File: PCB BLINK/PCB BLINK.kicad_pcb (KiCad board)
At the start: 2 copper layers, 74.9 x 74.9 mm, 6 parts, among them U2 HC-SR04, U3 ER_OLEDM0.91_1x-I2C

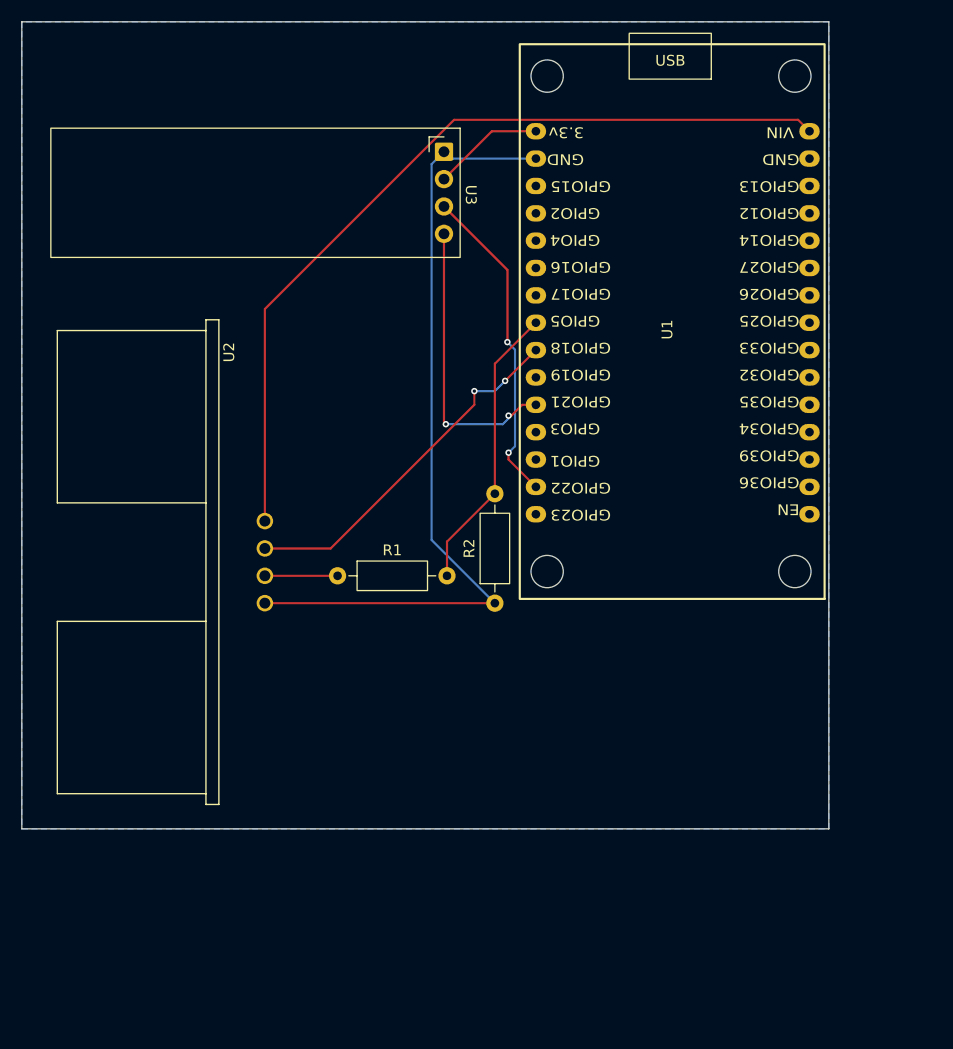
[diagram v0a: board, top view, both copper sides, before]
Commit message: case and pcb production
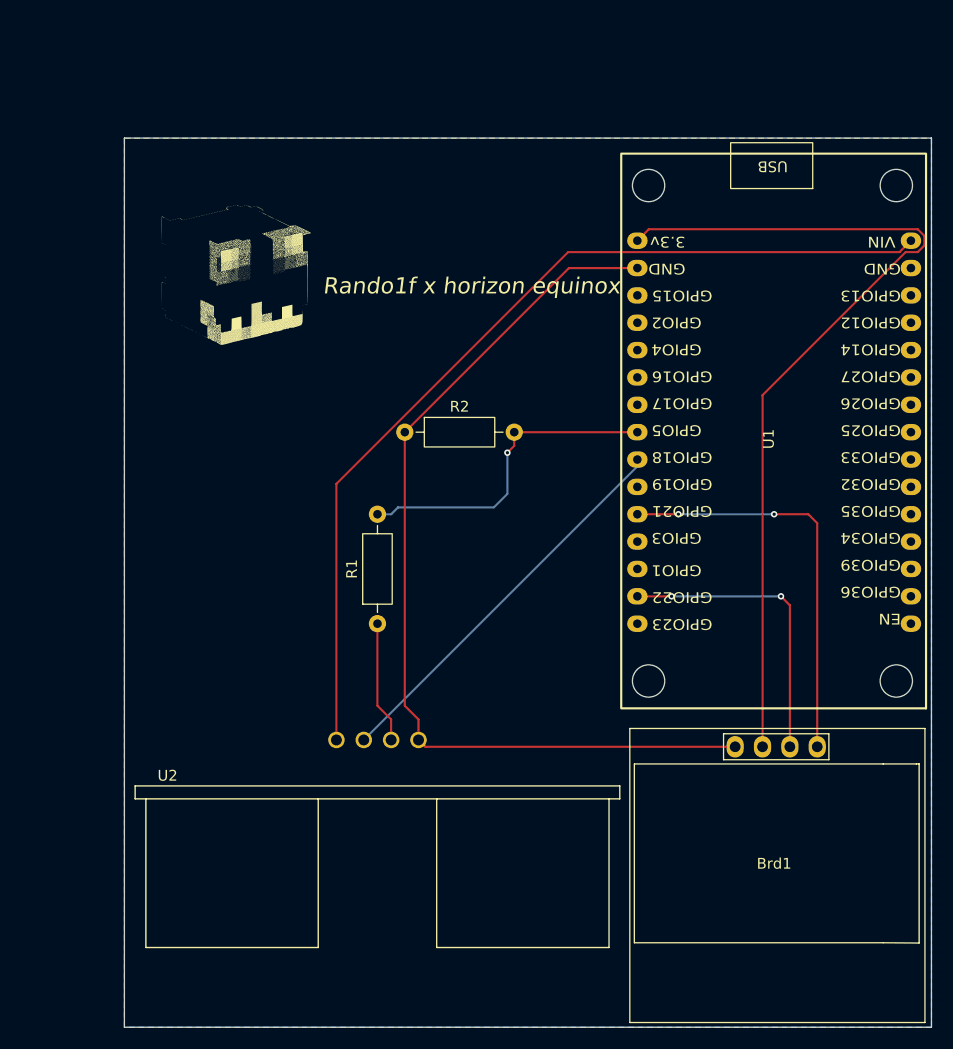
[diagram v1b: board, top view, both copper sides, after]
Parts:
- removed U3: ER_OLEDM0.91_1x-I2C, Display:ER_OLEDM0.91_1x-I2C
- added Brd1: SSD1306, SSD1306:128x64OLED, F.Cu at (183.5, 137.0)
- moved G*** 60.0 mm to (133.3, 82.5)
- moved U2 19.5 mm to (146.7, 125.7), turned to 0 degrees
- moved R2 17.9 mm to (149.2, 97.2), turned to 0 degrees
- moved U1 13.9 mm to (184.3, 96.4)
- moved R1 5.79 mm to (146.7, 114.9), turned to 90 degrees
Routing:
- net Net-(Brd1-VCC): track 10.4 -> 81.7 mm
- net GND: track 75.0 -> 86.7 mm
- net Net-(Brd1-SDA): track 27.0 -> 37.8 mm
- net Net-(U1-VIN): track 78.0 -> 86.5 mm
- net Net-(U2-ECHO): track 6.75 -> 11.3 mm
- net Net-(U1-GPIO5): track 26.9 -> 30.3 mm, vias 0 -> 1
- net Net-(U1-GPIO18): track 33.5 -> 36.6 mm, vias 2 -> 0
- net Net-(Brd1-SCL): track 30.1 -> 27.6 mm
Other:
- board size 74.9 x 74.9 mm -> 74.9 x 82.6 mm
- board text added: "Rando1f x horizon equinox"
